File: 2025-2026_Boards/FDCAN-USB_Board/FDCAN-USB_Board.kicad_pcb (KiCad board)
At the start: 2 copper layers, 50.5 x 34.8 mm, 61 parts, among them J2 Conn_01x03_Socket, J3 Conn_01x03_Socket, J4 Conn_01x03_Socket, J5 Conn_01x02_Pin, J6 Conn_ARM_JTAG_SWD_10, J7 USB4110-GF-A, U1 AMS1117-3.3, U2 USBLC6-2SC6, U3 STM32G474CETx, U4 TCAN1057AEV-Q1, U5 TCAN1057AEV-Q1, U6 TCAN1057AEV-Q1

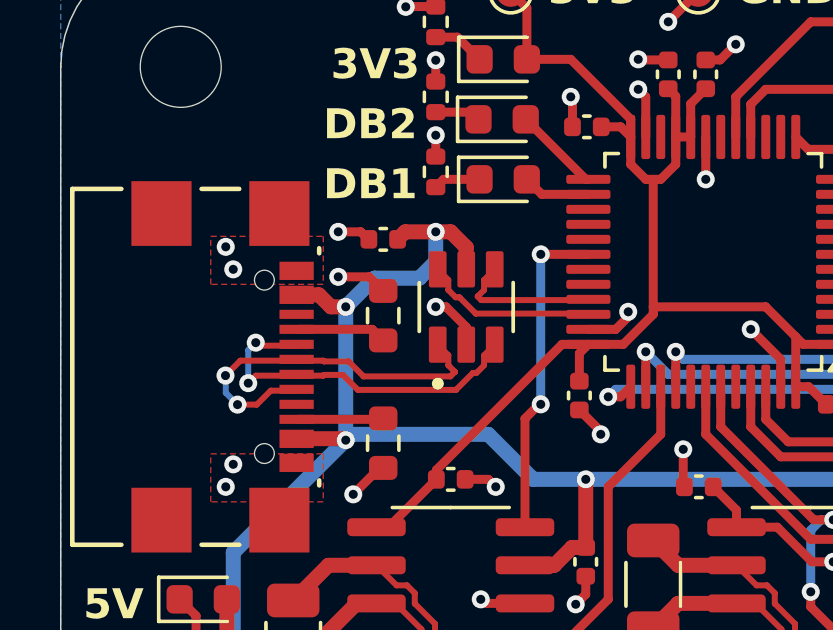
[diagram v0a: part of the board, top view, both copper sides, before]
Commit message: Final Design Reupload
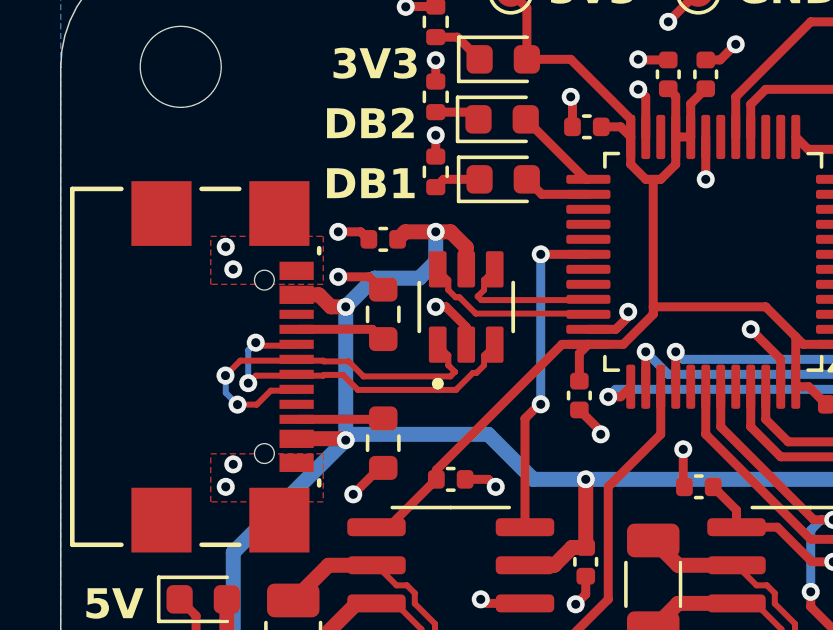
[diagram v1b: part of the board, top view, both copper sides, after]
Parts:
- C11: value 10n -> 100n
- R10, R11, R12, R14, R15, R5, R6, R7, R8, R9: value 1k -> 220
- turned R2 to 90 degrees
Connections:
- R2 pad 1: GND -> Net-(J7-CC1)
- R2 pad 2: Net-(J7-CC1) -> GND
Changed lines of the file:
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@@
 			)
 		)
-		(property "Value" "1k"
+		(property "Value" "220"
 			(at 0 1.17 0)
 			(layer "F.Fab")
@@
 			)
 		)
-		(property "Value" "1k"
+		(property "Value" "220"
 			(at 0 1.17 0)
 			(layer "F.Fab")
@@
 		)
 	)
+	(footprint "Resistor_SMD:R_0603_1608Metric"
+		(layer "F.Cu")
+		(at 85.75 62.25 90)
+		(descr "Resistor SMD 0603 (1608 Metric), square (rectangular) end terminal, IPC-7351 nominal, (Body size source: IPC-SM-782 page 72, https://www.pcb-3d.com/wordpress/wp-content/uploads/ipc-sm-782a_amendment_1_and_2.pdf), generated with kicad-footprint-generator")
+		(tags "resistor")
+		(property "Reference" "R2"
+			(at 0 -1.43 90)
+			(layer "F.SilkS")
+			(hide yes)
+			(effects
+				(font
+					(size 1 1)
+					(thickness 0.15)
+				)
+			)
+		)
+		(property "Value" "5.1k"
+			(at 0 1.43 90)
+			(layer "F.Fab")
+			(effects
+				(font
+					(size 1 1)
+					(thickness 0.15)
+				)
+			)
+		)
+		(property "Datasheet" "~"
+			(at 0 0 90)
+			(layer "F.Fab")
+			(hide yes)
+			(effects
+				(font
+					(size 1.27 1.27)
+					(thickness 0.15)
+				)
+			)
+		)
+		(property "Description" "Resistor, US symbol"
+			(at 0 0 90)
+			(layer "F.Fab")
+			(hide yes)
+			(effects
+				(font
+					(size 1.27 1.27)
+					(thickness 0.15)
+				)
+			)
+		)
+		(property ki_fp_filters "R_*")
+		(sheetname "/USB Power/")
+		(sheetfile "USB_Power.kicad_sch")
+		(attr smd)
+		(fp_line
+			(start -0.237258 -0.5225)
+			(end 0.237258 -0.5225)
+			(stroke
+				(width 0.12)
+				(type solid)
+			)
+			(layer "F.SilkS")
+		)
+		(fp_line
+			(start -0.237258 0.5225)
+			(end 0.237258 0.5225)
+			(stroke
+				(width 0.12)
+				(type solid)
+			)
+			(layer "F.SilkS")
+		)
+		(fp_line
+			(start 1.48 -0.73)
+			(end 1.48 0.73)
+			(stroke
+				(width 0.05)
+				(type solid)
+			)
+			(layer "F.CrtYd")
+		)
+		(fp_line
+			(start -1.48 -0.73)
+			(end 1.48 -0.73)
+			(stroke
+				(width 0.05)
+				(type solid)
+			)
+			(layer "F.CrtYd")
+		)
+		(fp_line
+			(start 1.48 0.73)
+			(end -1.48 0.73)
+			(stroke
+				(width 0.05)
+				(type solid)
+			)
+			(layer "F.CrtYd")
+		)
+		(fp_line
+			(start -1.48 0.73)
+			(end -1.48 -0.73)
+			(stroke
+				(width 0.05)
+				(type solid)
+			)
+			(layer "F.CrtYd")
+		)
+		(fp_line
+			(start 0.8 -0.4125)
+			(end 0.8 0.4125)
+			(stroke
+				(width 0.1)
+				(type solid)
+			)
+			(layer "F.Fab")
+		)
+		(fp_line
+			(start -0.8 -0.4125)
+			(end 0.8 -0.4125)
+			(stroke
+				(width 0.1)
+				(type solid)
+			)
+			(layer "F.Fab")
+		)
+		(fp_line
+			(start 0.8 0.4125)
+			(end -0.8 0.4125)
+			(stroke
+				(width 0.1)
+				(type solid)
+			)
+			(layer "F.Fab")
+		)
+		(fp_line
+			(start -0.8 0.4125)
+			(end -0.8 -0.4125)
+			(stroke
+				(width 0.1)
+				(type solid)
+			)
+			(layer "F.Fab")
+		)
+		(fp_text user "${REFERENCE}"
+			(at 0 0 90)
+			(layer "F.Fab")
+			(effects
+				(font
+					(size 0.4 0.4)
+					(thickness 0.06)
+				)
+			)
+		)
+		(pad "1" smd roundrect
+			(at -0.825 0 90)
+			(size 0.8 0.95)
+			(layers "F.Cu" "F.Mask" "F.Paste")
+			(roundrect_rratio 0.25)
+			(net 22 "Net-(J7-CC1)")
+			(pintype "passive")
+		)
+		(pad "2" smd roundrect
+			(at 0.825 0 90)
+			(size 0.8 0.95)
+			(layers "F.Cu" "F.Mask" "F.Paste")
+			(roundrect_rratio 0.25)
+			(net 1 "GND")
+			(pintype "passive")
+		)
+		(embedded_fonts no)
+		(model "${KICAD9_3DMODEL_DIR}/Resistor_SMD.3dshapes/R_0603_1608Metric.step"
+			(offset
+				(xyz 0 0 0)
+			)
+			(scale
+				(xyz 1 1 1)
+			)
+			(rotate
+				(xyz 0 0 0)
+			)
+		)
+	)
 	(footprint "Resistor_SMD:R_0402_1005Metric"
 		(layer "F.Cu")
@@
 			)
 		)
-		(property "Value" "1k"
+		(property "Value" "220"
 			(at 0 1.17 0)
 			(layer "F.Fab")
@@
 			)
 		)
-		(property "Value" "1k"
+		(property "Value" "220"
 			(at 0 1.17 0)
 			(layer "F.Fab")
@@
 		)
 	)
-	(footprint "Resistor_SMD:R_0603_1608Metric"
-		(layer "F.Cu")
-		(at 85.75 62.29375 -90)
-		(descr "Resistor SMD 0603 (1608 Metric), square (rectangular) end terminal, IPC-7351 nominal, (Body size source: IPC-SM-782 page 72, https://www.pcb-3d.com/wordpress/wp-content/uploads/ipc-sm-782a_amendment_1_and_2.pdf), generated with kicad-footprint-generator")
-		(tags "resistor")
-		(property "Reference" "R2"
-			(at 0 -1.43 90)
-			(layer "F.SilkS")
-			(hide yes)
-			(effects
-				(font
-					(size 1 1)
-					(thickness 0.15)
-				)
-			)
-		)
-		(property "Value" "5.1k"
-			(at 0 1.43 90)
-			(layer "F.Fab")
-			(hide yes)
-			(effects
-				(font
-					(size 1 1)
-					(thickness 0.15)
-				)
-			)
-		)
-		(property "Datasheet" "~"
-			(at 0 0 90)
-			(layer "F.Fab")
-			(hide yes)
-			(effects
-				(font
-					(size 1.27 1.27)
-					(thickness 0.15)
-				)
-			)
-		)
-		(property "Description" "Resistor, US symbol"
-			(at 0 0 90)
-			(layer "F.Fab")
-			(hide yes)
-			(effects
-				(font
-					(size 1.27 1.27)
-					(thickness 0.15)
-				)
-			)
-		)
-		(property ki_fp_filters "R_*")
-		(sheetname "/USB Power/")
-		(sheetfile "USB_Power.kicad_sch")
-		(attr smd)
-		(fp_line
-			(start -0.237258 0.5225)
-			(end 0.237258 0.5225)
-			(stroke
-				(width 0.12)
-				(type solid)
-			)
-			(layer "F.SilkS")
-		)
-		(fp_line
-			(start -0.237258 -0.5225)
-			(end 0.237258 -0.5225)
-			(stroke
-				(width 0.12)
-				(type solid)
-			)
-			(layer "F.SilkS")
-		)
-		(fp_line
-			(start -1.48 0.73)
-			(end -1.48 -0.73)
-			(stroke
-				(width 0.05)
-				(type solid)
-			)
-			(layer "F.CrtYd")
-		)
-		(fp_line
-			(start 1.48 0.73)
-			(end -1.48 0.73)
-			(stroke
-				(width 0.05)
-				(type solid)
-			)
-			(layer "F.CrtYd")
-		)
-		(fp_line
-			(start -1.48 -0.73)
-			(end 1.48 -0.73)
-			(stroke
-				(width 0.05)
-				(type solid)
-			)
-			(layer "F.CrtYd")
-		)
-		(fp_line
-			(start 1.48 -0.73)
-			(end 1.48 0.73)
-			(stroke
-				(width 0.05)
-				(type solid)
-			)
-			(layer "F.CrtYd")
-		)
-		(fp_line
-			(start -0.8 0.4125)
-			(end -0.8 -0.4125)
-			(stroke
-				(width 0.1)
-				(type solid)
-			)
-			(layer "F.Fab")
-		)
-		(fp_line
-			(start 0.8 0.4125)
-			(end -0.8 0.4125)
-			(stroke
-				(width 0.1)
-				(type solid)
-			)
-			(layer "F.Fab")
-		)
-		(fp_line
-			(start -0.8 -0.4125)
-			(end 0.8 -0.4125)
-			(stroke
-				(width 0.1)
-				(type solid)
-			)
-			(layer "F.Fab")
-		)
-		(fp_line
-			(start 0.8 -0.4125)
-			(end 0.8 0.4125)
-			(stroke
-				(width 0.1)
-				(type solid)
-			)
-			(layer "F.Fab")
-		)
-		(fp_text user "${REFERENCE}"
-			(at 0 0 90)
-			(layer "F.Fab")
-			(effects
-				(font
-					(size 0.4 0.4)
-					(thickness 0.06)
-				)
-			)
-		)
-		(pad "1" smd roundrect
-			(at -0.825 0 270)
-			(size 0.8 0.95)
-			(layers "F.Cu" "F.Mask" "F.Paste")
-			(roundrect_rratio 0.25)
-			(net 1 "GND")
-			(pintype "passive")
-		)
-		(pad "2" smd roundrect
-			(at 0.825 0 270)
-			(size 0.8 0.95)
-			(layers "F.Cu" "F.Mask" "F.Paste")
-			(roundrect_rratio 0.25)
-			(net 22 "Net-(J7-CC1)")
-			(pintype "passive")
-		)
-		(embedded_fonts no)
-		(model "${KICAD9_3DMODEL_DIR}/Resistor_SMD.3dshapes/R_0603_1608Metric.step"
-			(offset
-				(xyz 0 0 0)
-			)
-			(scale
-				(xyz 1 1 1)
-			)
-			(rotate
-				(xyz 0 0 0)
-			)
-		)
-	)
 	(footprint "Capacitor_SMD:C_0402_1005Metric"
 		(layer "F.Cu")
@@
 			)
 		)
-		(property "Value" "1k"
+		(property "Value" "220"
 			(at 0 1.17 0)
 			(layer "F.Fab")
@@
 			)
 		)
-		(property "Value" "1k"
+		(property "Value" "220"
 			(at 0 1.17 90)
 			(layer "F.Fab")
@@
 			)
 		)
-		(property "Value" "1k"
+		(property "Value" "220"
 			(at 0 1.17 90)
 			(layer "F.Fab")
@@
 			)
 		)
-		(property "Value" "1k"
+		(property "Value" "220"
 			(at 0 1.17 90)
 			(layer "F.Fab")
@@
 			)
 		)
-		(property "Value" "1k"
+		(property "Value" "220"
 			(at 0 1.17 0)
 			(layer "F.Fab")
@@
 			)
 		)
-		(property "Value" "1k"
+		(property "Value" "220"
 			(at 0 1.17 0)
 			(layer "F.Fab")
@@
 			)
 		)
-		(property "Value" "10n"
+		(property "Value" "100n"
 			(at 0 1.16 90)
 			(layer "F.Fab")
